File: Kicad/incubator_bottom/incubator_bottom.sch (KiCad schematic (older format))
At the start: 29 parts, among them J1 Conn_01x02, J2 Conn_02x03_Odd_Even, J3 RJ12, J4 Conn_01x05, J5 AudioJack3_SwitchTR, J6 AudioJack3_SwitchTR, Q1 ZXMS6004, U1 DS18B20Z, U2 DS18B20

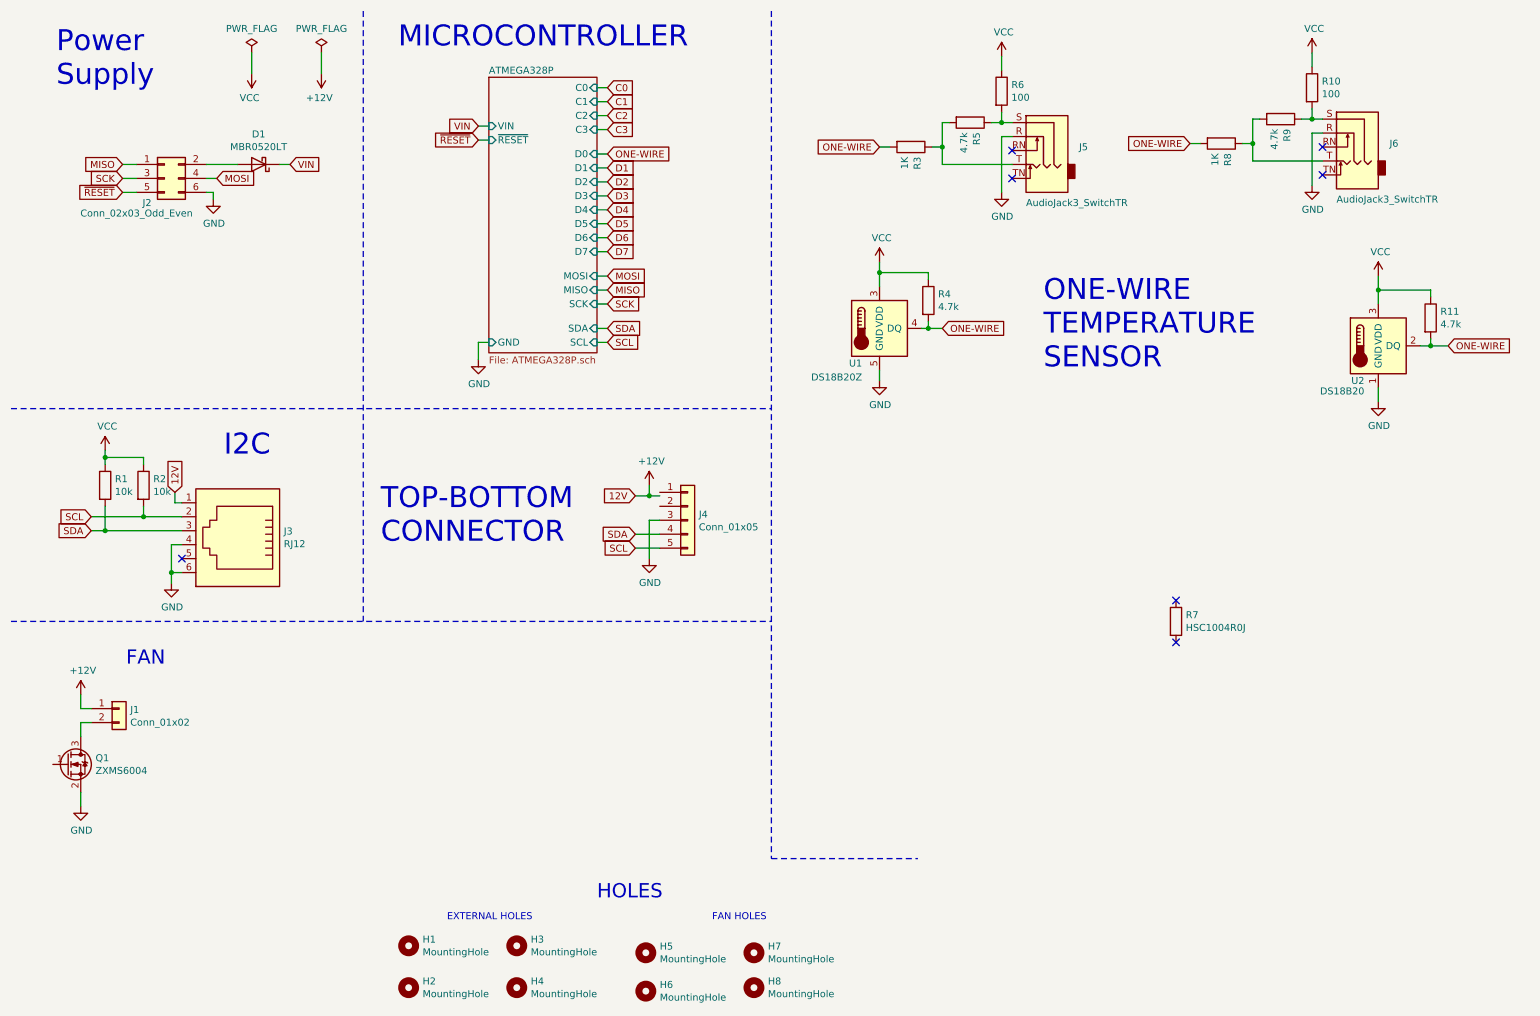
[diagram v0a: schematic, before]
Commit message: refactor: Kicad design updated
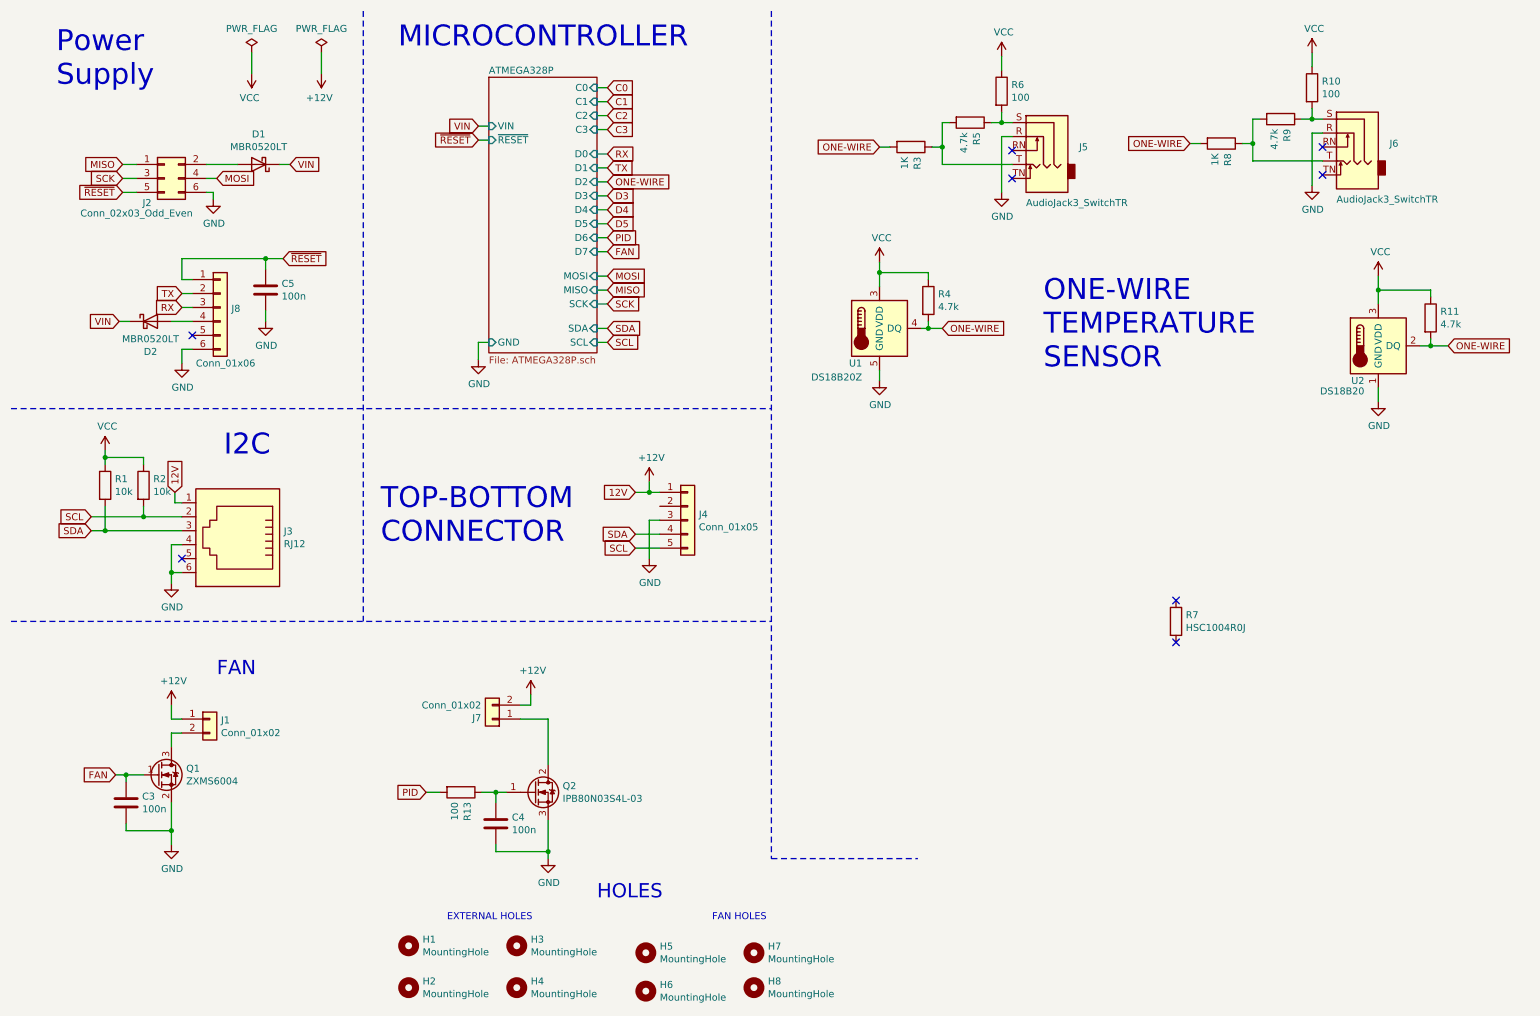
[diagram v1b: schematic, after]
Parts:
- added C3, C4, C5: 100n, Capacitor_SMD:C_0805_2012Metric_Pad1.18x1.45mm_HandSolder, symbol Device:C
- added D2: MBR0520LT, Diode_SMD:D_SOD-123, symbol Diode:MBR0520LT
- added J7: Conn_01x02, Connector_JST:JST_XH_B2B-XH-A_1x02_P2.50mm_Vertical, symbol Connector_Generic:Conn_01x02
- added J8: Conn_01x06, Connector_PinHeader_2.54mm:PinHeader_1x06_P2.54mm_Vertical, symbol Connector_Generic:Conn_01x06
- added Q2: IPB80N03S4L-03, Package_TO_SOT_SMD:TO-263-2, symbol Bertha_main:IPB80N03S4L-03
- added R13: 100, Resistor_SMD:R_0805_2012Metric_Pad1.20x1.40mm_HandSolder, symbol Device:R
- H5, H6, H7, H8: footprint MountingHole:MountingHole_3.2mm_M3 -> MountingHole:MountingHole_4.3mm_M4
- J1: footprint Connector_JST:JST_EH_B2B-EH-A_1x02_P2.50mm_Vertical -> Connector_JST:JST_XH_B2B-XH-A_1x02_P2.50mm_Vertical
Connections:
- net +12V: now also J4.1 (Pin_1), J7.2 (Pin_2)
- net GND: now also C3.2, C4.2, C5.2, J8.6 (Pin_6), Q2.3 (S)
- net VIN: now also D2.1 (K)
- net ~RESET: now also C5.1, J8.1 (Pin_1)
- net FAN: now reaches Q1.1 (G)
- net FAN: now also C3.1
- new net: J7.1 (Pin_1), Q2.2 (D)
- new net: C4.1, Q2.1 (G), R13.1
- new net: D2.2 (A), J8.4 (Pin_4)
- new net PID: R13.2
- new net RX: J8.3 (Pin_3)
- new net TX: J8.2 (Pin_2)
- no-connect marks 7 -> 8
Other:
- moved on the sheet: J1, Q1
